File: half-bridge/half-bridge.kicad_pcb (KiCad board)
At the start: 4 copper layers, 56 x 37 mm, 51 parts, among them J1 Conn_01x11_Pin, J2 Conn_01x11_Pin, J3 Conn_01x04_Pin, J4 Conn_01x04_Pin, J5 Conn_01x11_Pin, J6 Conn_01x11_Pin, J7 Conn_01x11_Pin, J8 Conn_01x11_Pin, Q1 GAN7R0-150LBE, Q2 GAN7R0-150LBE, U1 LMG1210

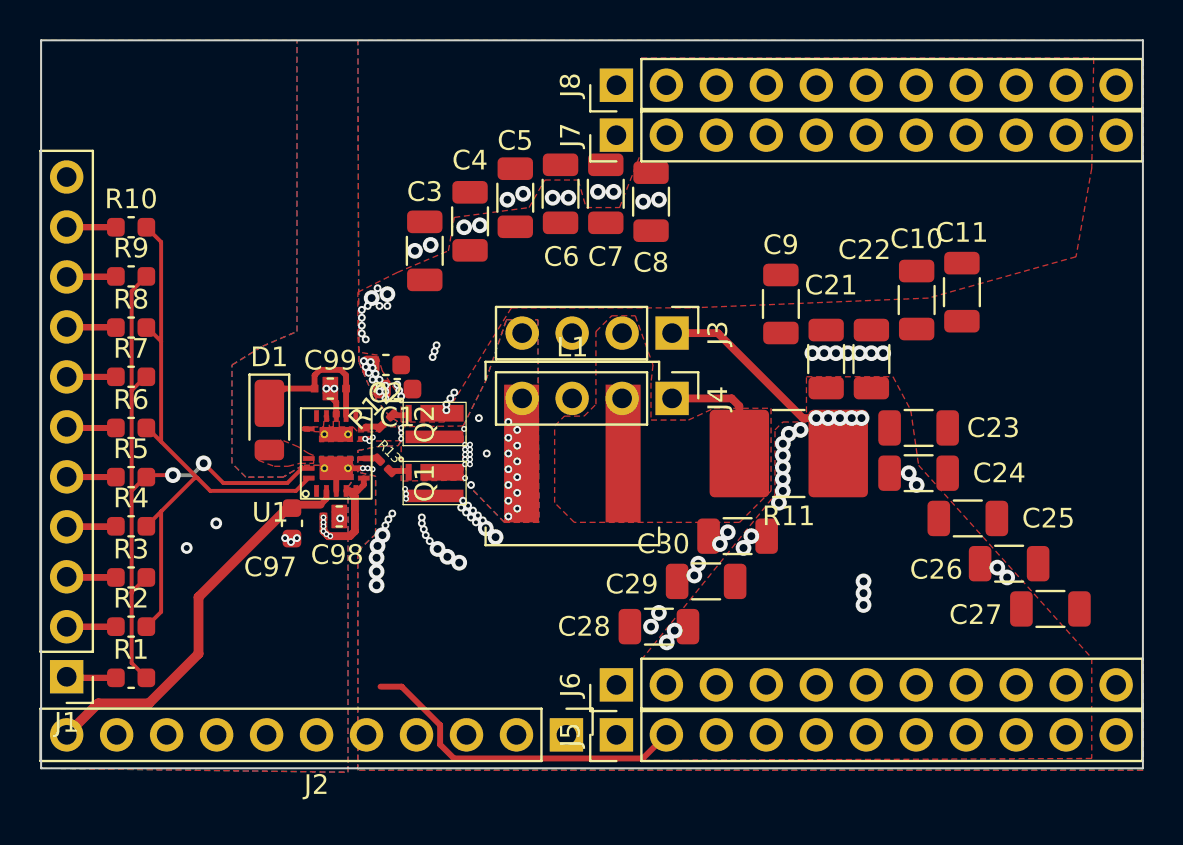
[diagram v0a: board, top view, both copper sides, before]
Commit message: Some changes
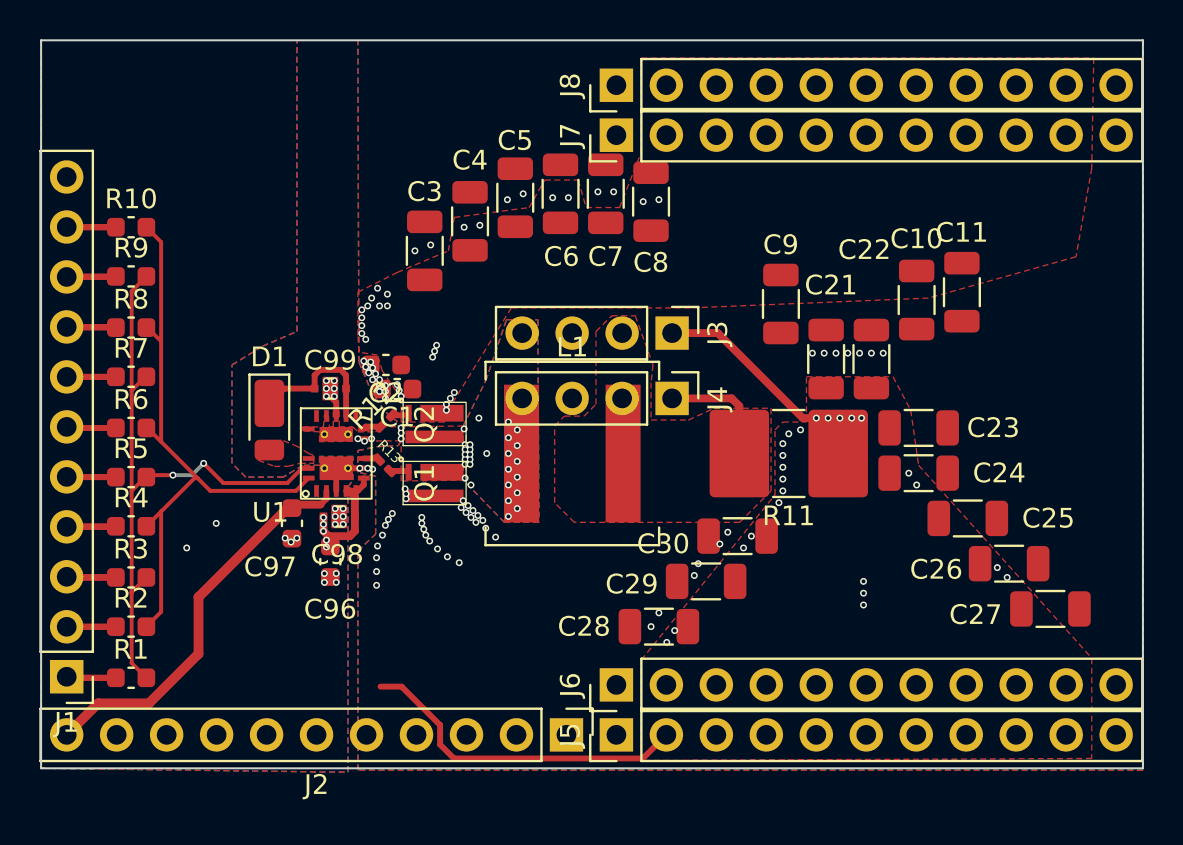
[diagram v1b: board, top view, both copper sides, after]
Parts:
- added C96: 10uF, Capacitor_SMD:C_0603_1608Metric, F.Cu at (127.7, 105.5)
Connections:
- net Net-(J3-Pin_1) renamed POWER_LOW
- net Vbus renamed POWER_HIGH
- J2 pad 1: unconnected-(J2-Pin_1-Pad1) -> Net-(J2-Pin_1)
- J2 pad 2: unconnected-(J2-Pin_2-Pad2) -> Net-(J2-Pin_2)
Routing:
- net Switch_node: vias 36 -> 40
- net Earth: vias 6 -> 15
- net +5V: vias 6 -> 5
